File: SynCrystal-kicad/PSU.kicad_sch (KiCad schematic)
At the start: 14 parts, among them U3 AP63205WU, U5 AP2210N-3.3TRG1

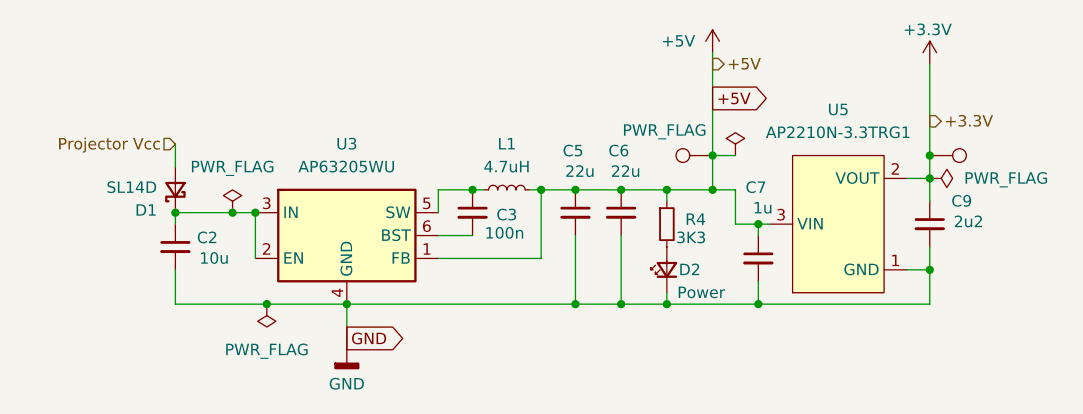
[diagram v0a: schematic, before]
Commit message: Projector PCB!
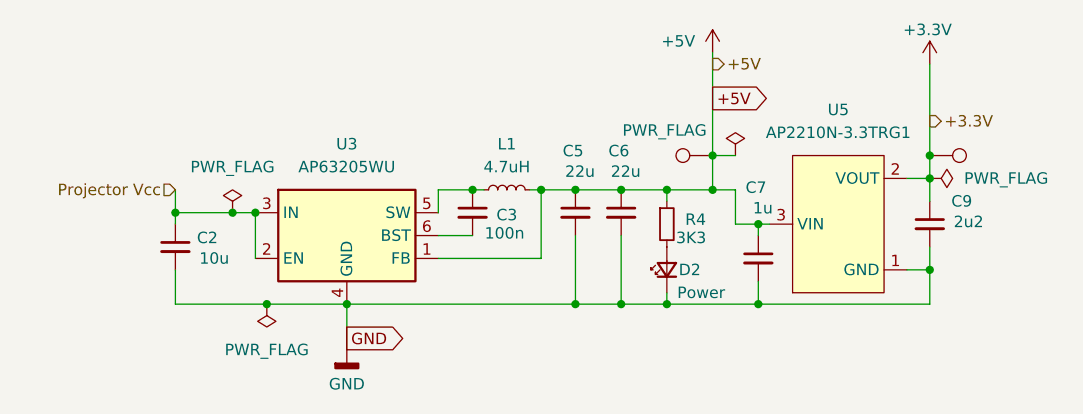
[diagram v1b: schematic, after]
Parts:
- removed D1: SL14D, Diode_SMD:D_SMA, symbol Device:D_Schottky_Small
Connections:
- net Projector Vcc: now also C2.1, U3.2 (EN), U3.3 (IN)
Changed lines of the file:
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@@
+	)
+	(junction
+		(at 87.63 73.66)
+		(diameter 0)
+		(color 0 0 0 0)
 	)
 	(junction
@@
 	)
 	(junction
-		(at 87.63 73.66)
-		(diameter 0)
-		(color 0 0 0 0)
-	)
-	(junction
 		(at 152.4 74.93)
 		(diameter 0)
@@
 	(wire
 		(pts
-			(xy 87.63 66.04) (xy 87.63 68.58)
+			(xy 87.63 71.12) (xy 87.63 73.66)
 		)
 		(stroke
@@
 	(hierarchical_label "Projector Vcc"
 		(shape input)
-		(at 87.63 66.04 180)
+		(at 87.63 71.12 180)
 		(effects
 			(font
@@
 					(unit 1)
 				)
-			)
-		)
-	)
-	(symbol
-		(lib_id "Device:D_Schottky_Small")
-		(at 87.63 71.12 90)
-		(unit 1)
-		(exclude_from_sim no)
-		(in_bom yes)
-		(on_board yes)
-		(dnp no)
-		(property "Reference" "D1"
-			(at 85.598 73.406 90)
-			(effects
-				(font
-					(size 1.27 1.27)
-				)
-				(justify left)
-			)
-		)
-		(property "Value" "SL14D"
-			(at 85.598 70.866 90)
-			(effects
-				(font
-					(size 1.27 1.27)
-				)
-				(justify left)
-			)
-		)
-		(property "Footprint" "Diode_SMD:D_SMA"
-			(at 87.63 71.12 90)
-			(effects
-				(font
-					(size 1.27 1.27)
-				)
-				(hide yes)
-			)
-		)
-		(property "Datasheet" "~"
-			(at 87.63 71.12 90)
-			(effects
-				(font
-					(size 1.27 1.27)
-				)
-				(hide yes)
-			)
-		)
-		(property "Description" "Schottky diode, small symbol"
-			(at 87.63 71.12 0)
-			(effects
-				(font
-					(size 1.27 1.27)
-				)
-				(hide yes)
-			)
-		)
-		(pin "2"
-		)
-		(pin "1"
-		)
-		(instances
-			(project "SynCrystal-kicad"
-				(path "/904e3c46-2ed3-4778-9ca9-733b218304b0/dbbd1505-7649-4218-add0-57fe64ba3603"
-					(reference "D1")
-					(unit 1)
-				)

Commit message: Starting to assign part numbers
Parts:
- removed C2: 10u, Capacitor_SMD:C_0603_1608Metric, symbol Device:C_Small
- removed C3: 100n, Capacitor_SMD:C_0603_1608Metric, symbol Device:C_Small
- removed C5, C6: 22u, Capacitor_SMD:C_0603_1608Metric, symbol Device:C_Small
- removed C7: 1u, Capacitor_SMD:C_0603_1608Metric, symbol Device:C_Small
- removed C9: 2u2, Capacitor_SMD:C_0603_1608Metric, symbol Device:C_Small
- removed D2: Power, LED_SMD:LED_0805_2012Metric, symbol Device:LED_Small
- removed L1: 4.7uH, easyEDA:IND-SMD_L3.0-W3.0, symbol Device:L_Small
- removed R4: 3K3, Resistor_SMD:R_0603_1608Metric, symbol Device:R_Small
- removed TP7: 5V, TestPoint:TestPoint_Pad_D1.0mm, symbol Peacemans Teile:TestPoint_named
- removed TP8: 3V3, TestPoint:TestPoint_Pad_D1.0mm, symbol Peacemans Teile:TestPoint_named
- removed U3: AP63205WU, Package_TO_SOT_SMD:TSOT-23-6, symbol Regulator_Switching:AP63205WU
- removed U5: AP2210N-3.3TRG1, Package_TO_SOT_SMD:SOT-23-3, symbol easyEDA:AP2210N-3.3TRG1
